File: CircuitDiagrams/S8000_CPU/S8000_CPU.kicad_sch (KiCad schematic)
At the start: 0 parts

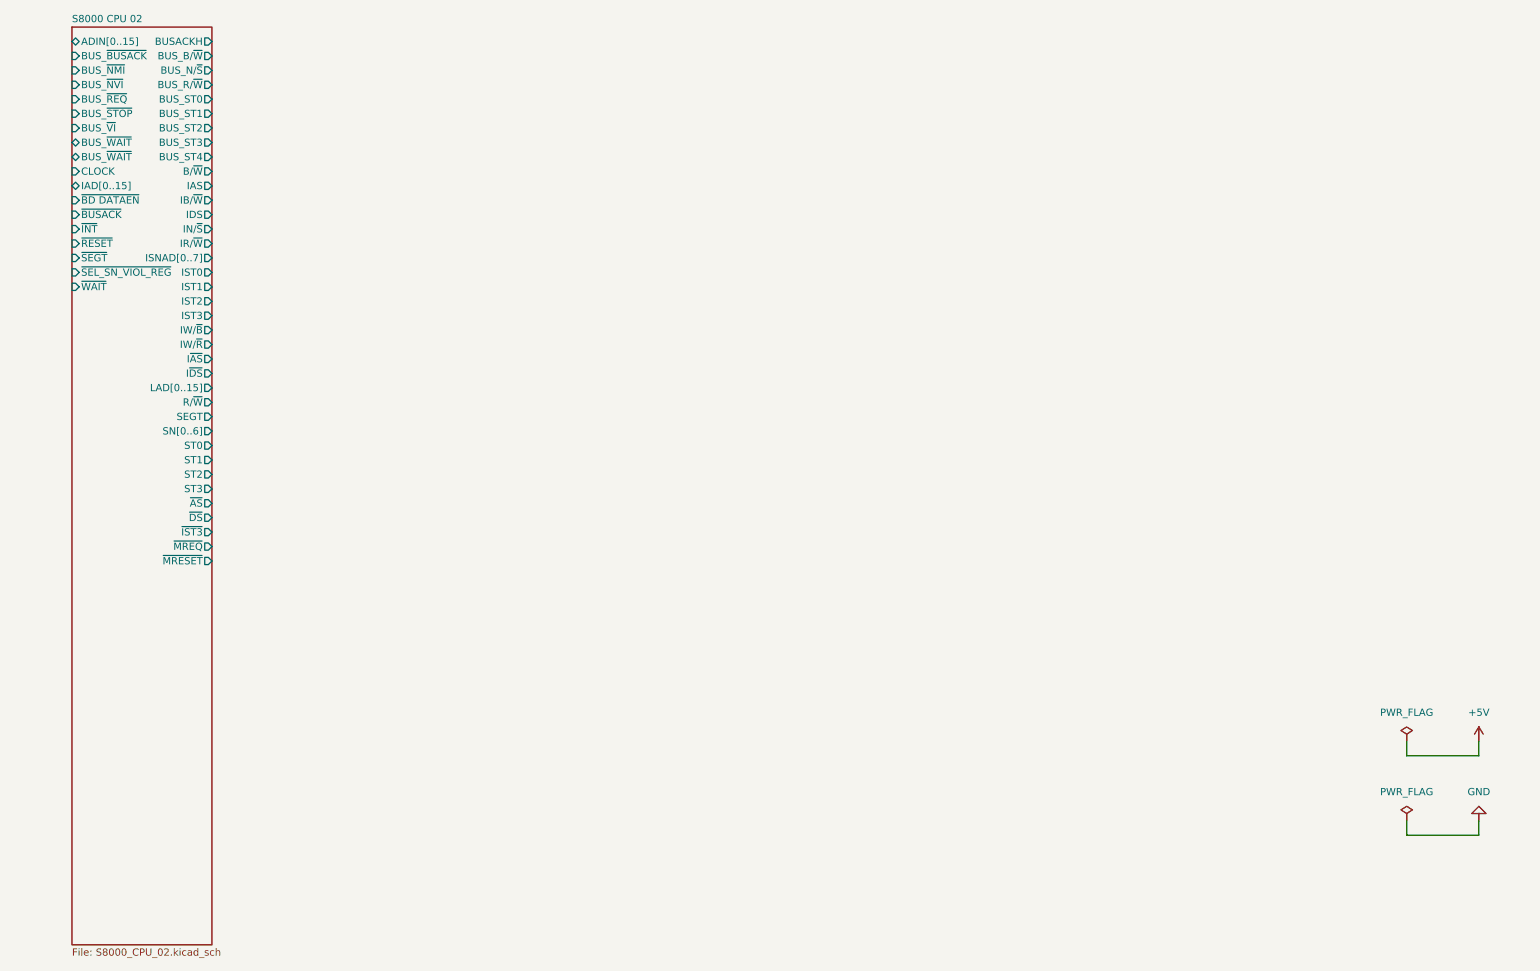
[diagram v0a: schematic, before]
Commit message: S8000 CPU schematics Page 3
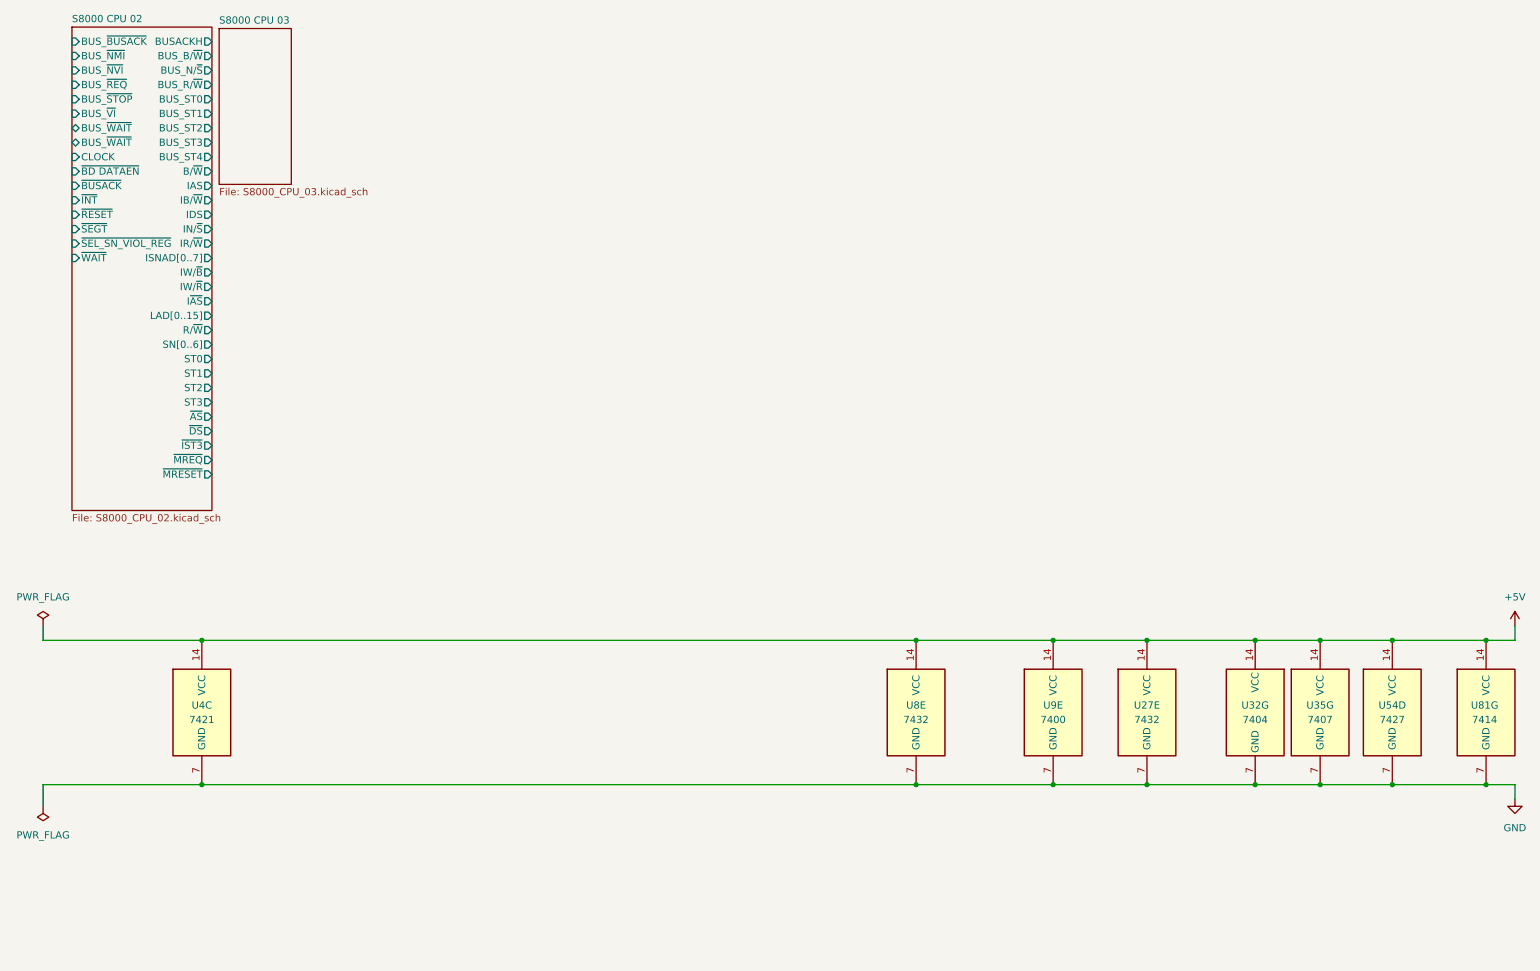
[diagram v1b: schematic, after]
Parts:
- added U27, U8: 7432, Package_DIP:DIP-14_W7.62mm, symbol 74xx:74LS32
- added U32: 7404, Package_DIP:DIP-14_W7.62mm, symbol 74xx:74LS04
- added U35: 7407, Package_DIP:DIP-14_W7.62mm, symbol 74xx:74LS07
- added U4: 7421, Package_DIP:DIP-14_W7.62mm, symbol 74xx:74LS21
- added U54: 7427, Package_DIP:DIP-14_W7.62mm, symbol 74xx:74LS27
- added U81: 7414, Package_DIP:DIP-14_W7.62mm, symbol 74xx:74LS14
- added U9: 7400, Package_DIP:DIP-14_W7.62mm, symbol 74xx:74LS00
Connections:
- net +5V: now also U27.14 (VCC), U32.14 (VCC), U35.14 (VCC), U4.14 (VCC), U54.14 (VCC), U8.14 (VCC), U81.14 (VCC), U9.14 (VCC)
- net GND: now also U27.7 (GND), U32.7 (GND), U35.7 (GND), U4.7 (GND), U54.7 (GND), U8.7 (GND), U81.7 (GND), U9.7 (GND)
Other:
- added sheet S8000 CPU 03 (S8000_CPU_03.kicad_sch)
- sheet S8000 CPU 02 ports: added none; removed ADIN[0..15], IAD[0..15], IST0, IST1, IST2, IST3, I~{DS}, SEGT

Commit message: Add Page 4
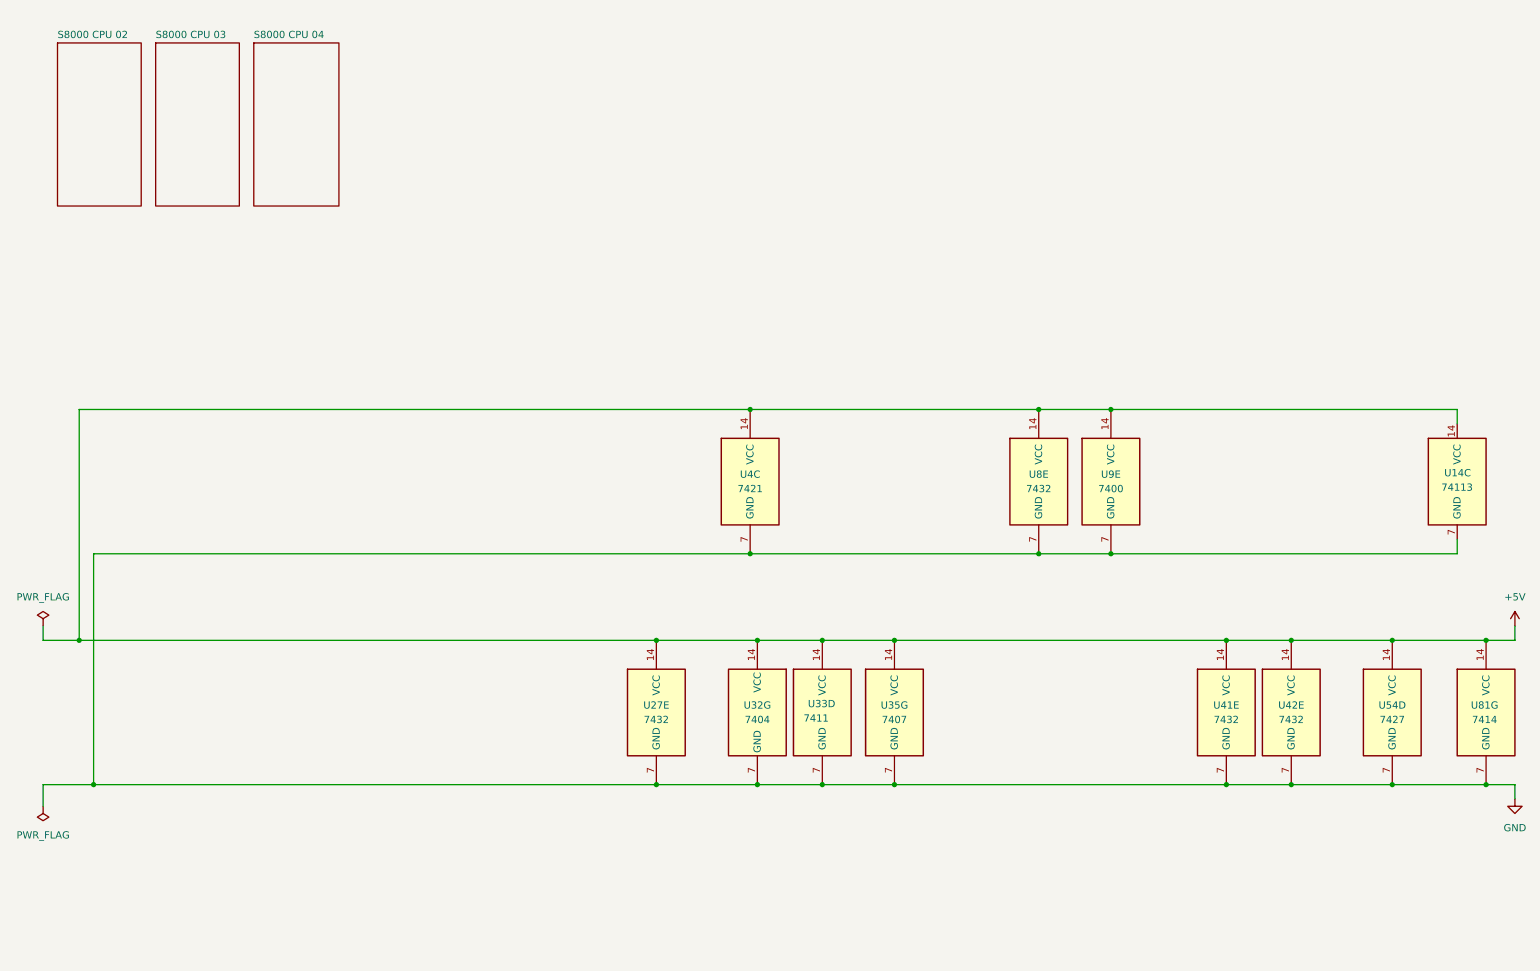
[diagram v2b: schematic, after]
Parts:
- added U14: 74113, Package_DIP:DIP-14_W7.62mm, symbol 74xx:74LS113
- added U33: 7411, Package_DIP:DIP-14_W7.62mm, symbol 74xx:74LS11
- added U41, U42: 7432, Package_DIP:DIP-14_W7.62mm, symbol 74xx:74LS32
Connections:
- net +5V: now also U14.14 (VCC), U33.14 (VCC), U41.14 (VCC), U42.14 (VCC)
- net GND: now also U14.7 (GND), U33.7 (GND), U41.7 (GND), U42.7 (GND)
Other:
- added sheet S8000 CPU 04 (S8000_CPU_04.kicad_sch)
- sheet S8000 CPU 02 ports: added none; removed BUSACKH, BUS_B/~{W}, BUS_N/~{S}, BUS_R/~{W}, BUS_ST0, BUS_ST1, BUS_ST2, BUS_ST3, BUS_ST4, BUS_~{BUSACK}, BUS_~{NMI}, BUS_~{NVI}, BUS_~{REQ}, BUS_~{STOP}, BUS_~{VI}, BUS_~{WAIT}, B/~{W}, CLOCK, IAS, IB/~{W}, IDS, IN/~{S}, IR/~{W}, ISNAD[0..7], IW/~{B}, IW/~{R}, I~{AS}, LAD[0..15], R/~{W}, SN[0..6], ST0, ST1, ST2, ST3, ~{AS}, ~{BD DATAEN}, ~{BUSACK}, ~{DS}, ~{INT}, ~{IST3}, ~{MREQ}, ~{MRESET}, ~{RESET}, ~{SEGT}, ~{SEL_SN_VIOL_REG}, ~{WAIT}
- moved on the sheet: U27E, U32G, U35G
